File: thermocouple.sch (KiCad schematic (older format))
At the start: 40 parts, among them CON1 AVR-ISP-6, IC1 SP3485CN, IC2 ATMEGA88-A, P1 CONN_2, P2 CONN_4, U1 AD8237, U2 TC1047, U3 7805, U4 LM358, X1 CRYSTAL

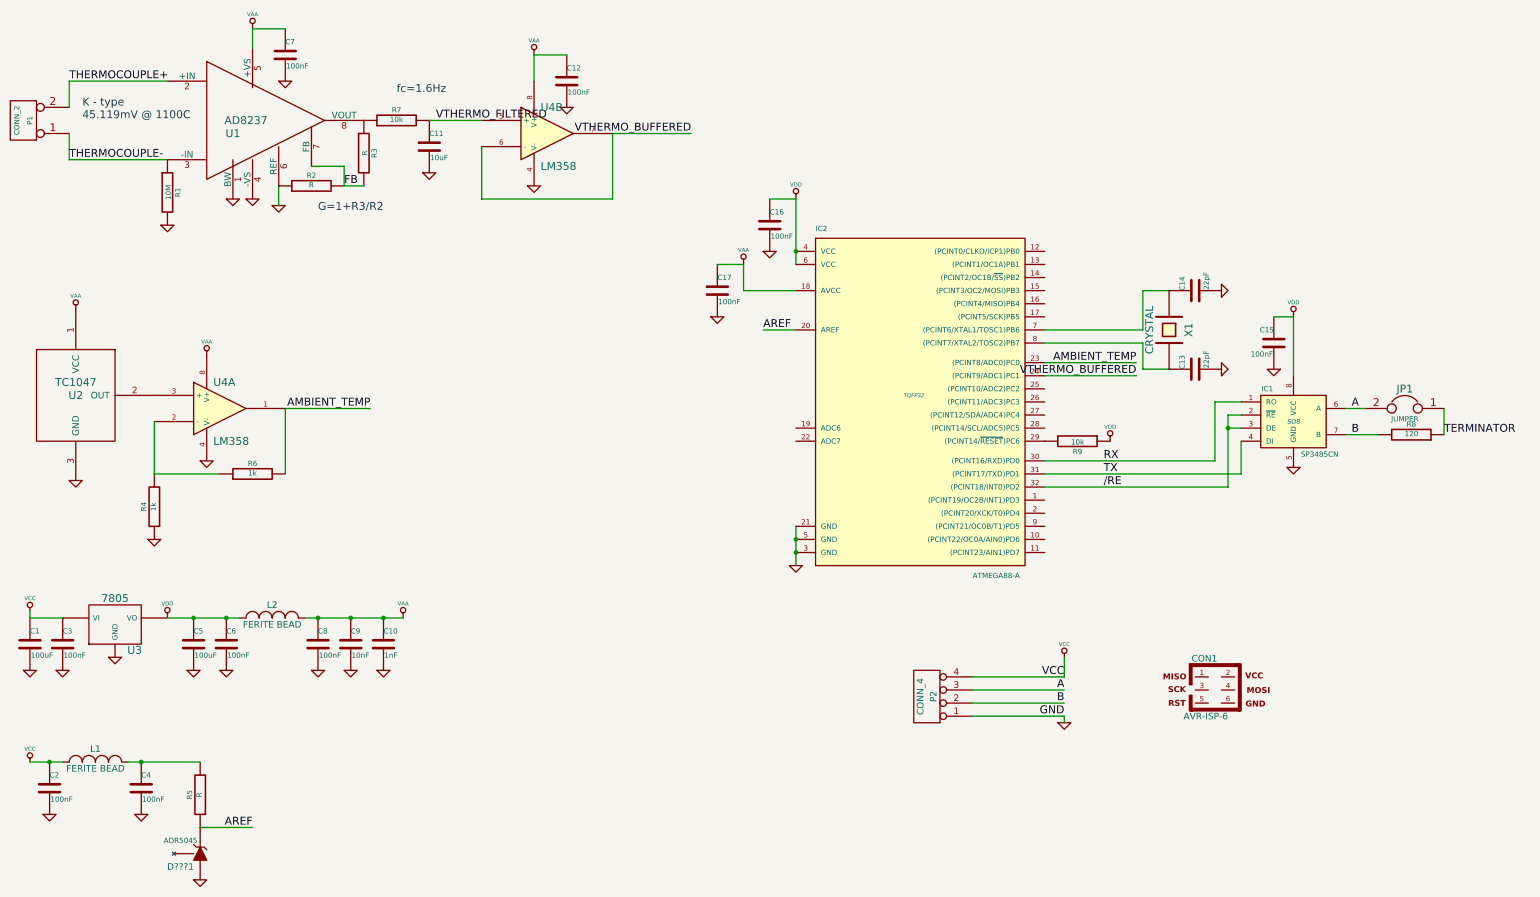
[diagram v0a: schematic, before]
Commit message: blah
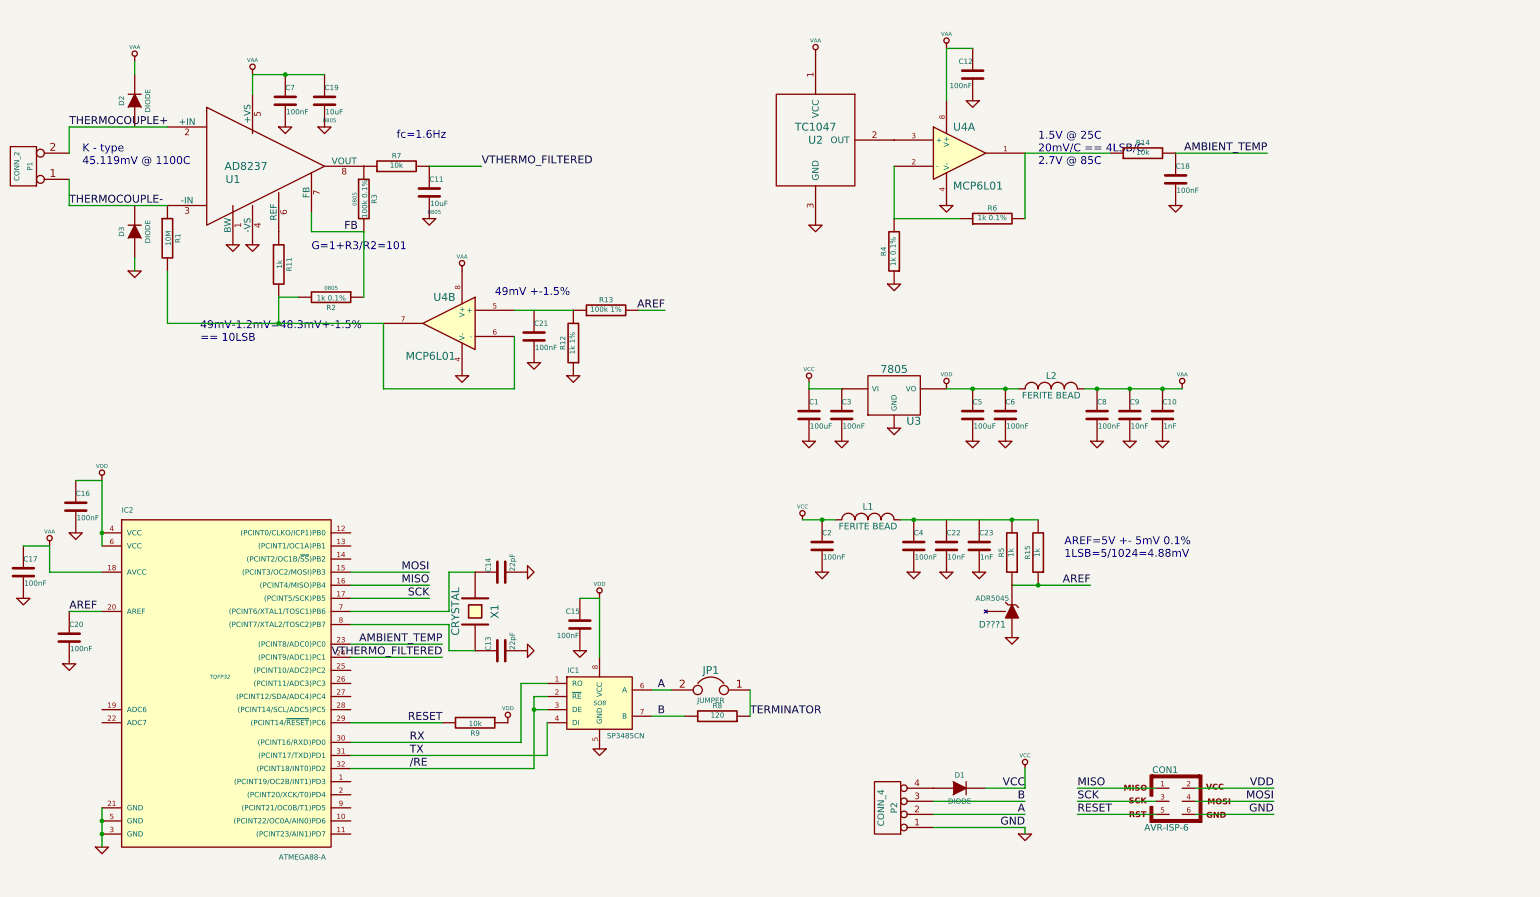
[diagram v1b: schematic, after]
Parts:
- added C18, C20, C21: 100nF, ~, symbol C
- added C19: 10uF, 0805, symbol C
- added C22: 10nF, ~, symbol C
- added C23: 1nF, ~, symbol C
- added D1, D2, D3: DIODE, ~, symbol DIODE
- added R11, R15: 1k, ~, symbol R
- added R12: 1k 1%, ~, symbol R
- added R13: 100k 1%, ~, symbol R
- added R14: 10k, ~, symbol R
- C11: footprint ~ -> 0805
- R2: value R -> 1k 0.1%; footprint ~ -> 0805
- R3: value R -> 100k 0.1%; footprint ~ -> 0805
- R4, R6: value 1k -> 1k 0.1%
- R5: value R -> 1k
- U4: value LM358 -> MCP6L01
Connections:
- net A: now also P2.2 (P2); no longer P2.3 (P3)
- net AMBIENT_TEMP: now also C18.1, R14.2; no longer R6.2, U4.1
- net AREF: now also C20.1, R13.2, R15.1
- net B: now also P2.3 (P3); no longer P2.2 (P2)
- net FB: now also R2.1; no longer R2.2
- net GND: now also CON1.6, C18.2, C19.2, C20.2, C21.2, C22.2, C23.2, D3.1 (A), R12.1; no longer R1.2, R2.1, U1.6 (REF)
- net VAA: now also C19.1, D2.2 (K)
- net VCC: now also D1.2 (K); no longer P2.4 (P4)
- net VDD: now also CON1.2
- net VTHERMO_FILTERED: now also IC2.24 ((PCINT9/ADC1)PC1); no longer U4.5 (+)
- net at C4.1, L1.2, R5.2: now also R15.2
- net RESET: now reaches IC2.29 ((PCINT14/~RESET~)PC6), R9.2
- net RESET: now also CON1.5
- net MISO: now reaches CON1.1
- net MISO: now also IC2.16 ((PCINT4/MISO)PB4)
- net SCK: now reaches CON1.3
- net SCK: now also IC2.17 ((PCINT5/SCK)PB5)
- net MOSI: now reaches CON1.4
- net MOSI: now also IC2.15 ((PCINT3/OC2/MOSI)PB3)
- net VTHERMO_BUFFERED: no longer names the net of U4.6 (-), U4.7
- net VTHERMO_BUFFERED: now also R1.2, R2.2, R11.2; no longer IC2.24 ((PCINT9/ADC1)PC1)
- new net: R11.1, U1.6 (REF)
- new net: R14.1, R6.2, U4.1
- new net: R12.2, R13.1, U4.5 (+)
- new net: D1.1 (A), P2.4 (P4)
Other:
- note added: "1.5V @ 25C\n20mV/C == 4LSB/C\n2.7V @ 85C"
- note added: "49mV +-1.5%"
- note added: "49mV-1.2mV=48.3mV+-1.5% \n== 10LSB"
- note added: "AREF=5V +- 5mV 0.1%\n1LSB=5/1024=4.88mV"
- note added: "G=1+R3/R2=101\n"
- note removed: "G=1+R3/R2\n"
- moved on the sheet: C1, C10, C11, C12, C13, C14, C15, C16, C17, C2, C3, C4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
